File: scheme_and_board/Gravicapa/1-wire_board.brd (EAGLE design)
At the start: 33.3 x 12.1 mm, 10 parts, among them IC1 DS18B20

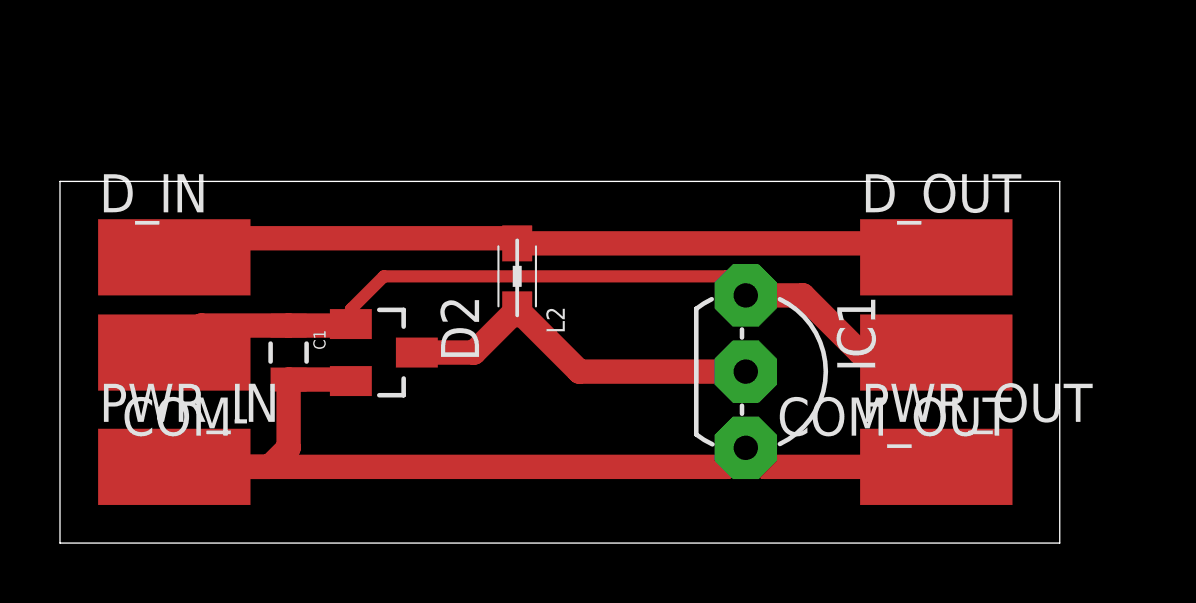
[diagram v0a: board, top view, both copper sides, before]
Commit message: �������� ����� ������������, ������� ��� ���������� � ������ ����������� ��� ������
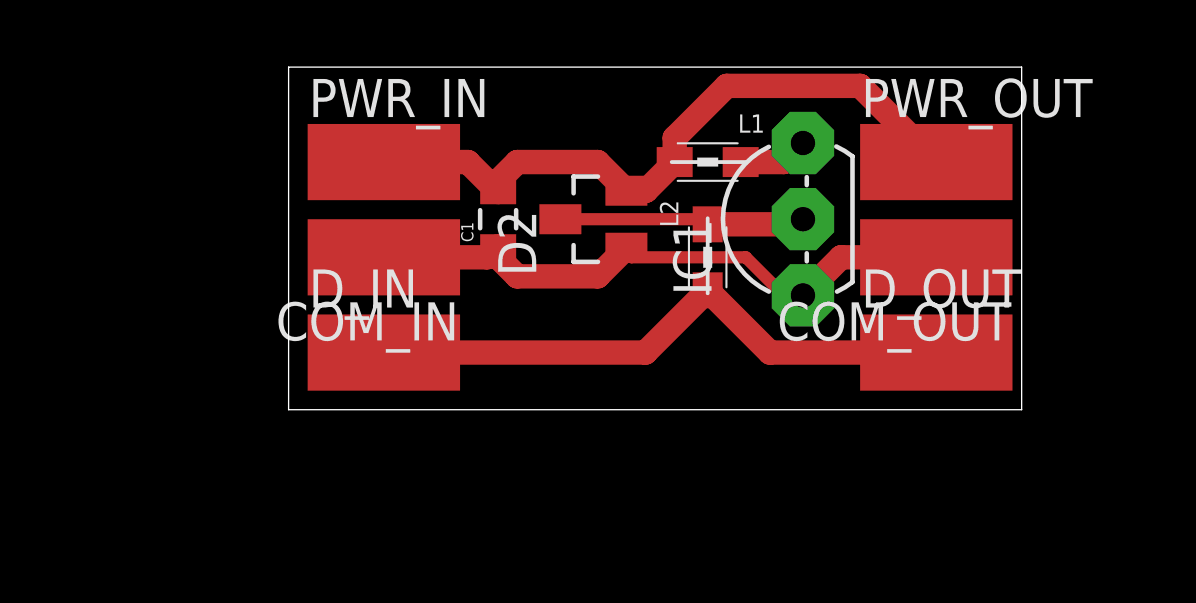
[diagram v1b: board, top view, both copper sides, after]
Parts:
- removed COM-: GND, wirepad:SMD2,54-5,08
- added COM_IN: GND, wirepad:SMD2,54-5,08
- added L1: BLM, wuerth-elektronik:0805
- moved PWR_IN 12.3 mm to (10.8, 12.7)
- moved PWR_OUT 10.2 mm to (29.2, 12.7)
- moved C1 8.28 mm to (14.6, 10.8), turned to 90 degrees
- moved D2 8.28 mm to (17.8, 10.8), turned to 90 degrees
- moved D_IN 7.67 mm to (10.8, 6.35)
- moved L2 6.38 mm to (21.6, 9.53), turned to 270 degrees
- moved IC1 5.43 mm to (24.8, 10.8), turned to 90 degrees
- moved COM_OUT 3.18 mm to (29.2, 9.53)
- moved D_OUT 3.18 mm to (29.2, 6.35)
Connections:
- new net N$4: C1.2, D2.2, L1.2, PWR_IN.1, PWR_OUT.1
- net N$3: now also COM_IN.1; no longer COM-.1
- net N$5: now also L1.1; no longer C1.2, D2.2, PWR_IN.1, PWR_OUT.1
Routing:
- net N$5: track 34.4 -> 2.34 mm
- net N$4: track 0.00 -> 22.8 mm
- net N$3: track 30.0 -> 21.1 mm
- net N$2: track 25.9 -> 20.1 mm
- net N$1: track 12.4 -> 8.23 mm
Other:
- board size 33.3 x 12.1 mm -> 24.4 x 11.4 mm
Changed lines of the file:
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@@
 <board>
 <plain>
-<wire x1="0" y1="0" x2="33.325" y2="0" width="0" layer="20"/>
-<wire x1="33.325" y1="0" x2="33.325" y2="12.055" width="0" layer="20"/>
-<wire x1="33.325" y1="12.055" x2="0" y2="12.055" width="0" layer="20"/>
-<wire x1="0" y1="12.055" x2="0" y2="0" width="0" layer="20"/>
+<wire x1="7.62" y1="4.445" x2="32.055" y2="4.445" width="0" layer="20"/>
+<wire x1="32.055" y1="4.445" x2="32.055" y2="15.865" width="0" layer="20"/>
+<wire x1="32.055" y1="15.865" x2="7.62" y2="15.865" width="0" layer="20"/>
+<wire x1="7.62" y1="15.865" x2="7.62" y2="4.445" width="0" layer="20"/>
 </plain>
 <attributes>
@@
 </autorouter>
 <elements>
-<element name="IC1" library="GravicapaLib" package="TO92-" value="DS18B20" x="22.86" y="5.715" rot="R270"/>
-<element name="L2" library="wuerth-elektronik" package="0805" value="BLM" x="15.24" y="8.89" rot="R90"/>
-<element name="D_IN" library="wirepad" package="SMD2,54-5,08" value="1-Wire" x="3.81" y="9.525" rot="R270"/>
-<element name="PWR_IN" library="wirepad" package="SMD2,54-5,08" value="VCC" x="3.81" y="2.54" rot="R270"/>
-<element name="COM-" library="wirepad" package="SMD2,54-5,08" value="GND" x="3.81" y="6.35" rot="R90"/>
-<element name="PWR_OUT" library="wirepad" package="SMD2,54-5,08" value="VCC" x="29.21" y="2.54" rot="R270"/>
-<element name="D_OUT" library="wirepad" package="SMD2,54-5,08" value="1-Wire" x="29.21" y="9.525" rot="R270"/>
-<element name="COM_OUT" library="wirepad" package="SMD2,54-5,08" value="GND" x="29.21" y="6.35" rot="R90"/>
-<element name="D2" library="GravicapaLib" package="SOT23" value="BAV199" x="10.795" y="6.35" rot="R270"/>
-<element name="C1" library="GravicapaLib" package="0805" value="0.1uF" x="7.62" y="6.35" rot="R270"/>
+<element name="IC1" library="GravicapaLib" package="TO92-" value="DS18B20" x="24.765" y="10.795" rot="R90"/>
+<element name="L2" library="wuerth-elektronik" package="0805" value="BLM" x="21.59" y="9.525" rot="R270"/>
+<element name="D_IN" library="wirepad" package="SMD2,54-5,08" value="1-Wire" x="10.795" y="6.35" rot="R270"/>
+<element name="PWR_IN" library="wirepad" package="SMD2,54-5,08" value="VCC" x="10.795" y="12.7" rot="R270"/>
+<element name="COM_IN" library="wirepad" package="SMD2,54-5,08" value="GND" x="10.795" y="9.525" rot="R90"/>
+<element name="PWR_OUT" library="wirepad" package="SMD2,54-5,08" value="VCC" x="29.21" y="12.7" rot="R270"/>
+<element name="D_OUT" library="wirepad" package="SMD2,54-5,08" value="1-Wire" x="29.21" y="6.35" rot="R270"/>
+<element name="COM_OUT" library="wirepad" package="SMD2,54-5,08" value="GND" x="29.21" y="9.525" rot="R90"/>
+<element name="D2" library="GravicapaLib" package="SOT23" value="BAV199" x="17.78" y="10.795" rot="R90"/>
+<element name="C1" library="GravicapaLib" package="0805" value="0.1uF" x="14.605" y="10.795" rot="R90"/>
+<element name="L1" library="wuerth-elektronik" package="0805" value="BLM" x="21.59" y="12.7" rot="R180"/>
 </elements>
 <signals>
@@
 <contactref element="IC1" pad="2"/>
 <contactref element="D2" pad="3"/>
-<wire x1="22.86" y1="5.715" x2="17.315" y2="5.715" width="0.8128" layer="1"/>
-<wire x1="17.315" y1="5.715" x2="15.24" y2="7.79" width="0.8128" layer="1"/>
-<wire x1="11.895" y1="6.35" x2="13.8" y2="6.35" width="0.8128" layer="1"/>
-<wire x1="13.8" y1="6.35" x2="15.24" y2="7.79" width="0.8128" layer="1"/>
+<wire x1="16.68" y1="10.795" x2="21.42" y2="10.795" width="0.4064" layer="1"/>
+<wire x1="21.42" y1="10.795" x2="21.59" y2="10.625" width="0.4064" layer="1"/>
+<wire x1="21.59" y1="10.625" x2="24.595" y2="10.625" width="0.8128" layer="1"/>
+<wire x1="24.595" y1="10.625" x2="24.765" y2="10.795" width="0.4064" layer="1"/>
 </signal>
 <signal name="N$5">
-<contactref element="PWR_OUT" pad="1"/>
 <contactref element="IC1" pad="3"/>
-<wire x1="22.86" y1="3.175" x2="23.495" y2="2.54" width="0.8128" layer="1"/>
-<wire x1="23.495" y1="2.54" x2="29.21" y2="2.54" width="0.8128" layer="1"/>
-<contactref element="PWR_IN" pad="1"/>
-<contactref element="D2" pad="2"/>
-<contactref element="C1" pad="2"/>
-<wire x1="7.62" y1="5.45" x2="9.645" y2="5.45" width="0.8128" layer="1"/>
-<wire x1="9.645" y1="5.45" x2="9.695" y2="5.4" width="0.8128" layer="1"/>
-<wire x1="3.81" y1="2.54" x2="22.225" y2="2.54" width="0.8128" layer="1"/>
-<wire x1="22.225" y1="2.54" x2="22.86" y2="3.175" width="0.8128" layer="1"/>
-<wire x1="3.81" y1="2.54" x2="6.985" y2="2.54" width="0.8128" layer="1"/>
-<wire x1="6.985" y1="2.54" x2="7.62" y2="3.175" width="0.8128" layer="1"/>
-<wire x1="7.62" y1="3.175" x2="7.62" y2="5.45" width="0.8128" layer="1"/>
+<contactref element="L1" pad="1"/>
+<wire x1="22.69" y1="12.7" x2="24.13" y2="12.7" width="0.8128" layer="1"/>
+<wire x1="24.13" y1="12.7" x2="24.765" y2="13.335" width="0.8128" layer="1"/>
 </signal>
 <signal name="N$3">
-<contactref element="COM-" pad="1"/>
+<contactref element="COM_IN" pad="1"/>
 <contactref element="IC1" pad="1"/>
 <contactref element="COM_OUT" pad="1"/>
 <contactref element="D2" pad="1"/>
 <contactref element="C1" pad="1"/>
-<wire x1="5.08" y1="6.35" x2="5.715" y2="6.985" width="1.016" layer="1"/>
-<wire x1="29.21" y1="6.35" x2="26.67" y2="6.35" width="0.8128" layer="1"/>
-<wire x1="26.67" y1="6.35" x2="24.765" y2="8.255" width="0.8128" layer="1"/>
-<wire x1="24.765" y1="8.255" x2="22.86" y2="8.255" width="0.8128" layer="1"/>
-<wire x1="3.81" y1="6.35" x2="5.08" y2="6.35" width="0.8128" layer="1"/>
-<wire x1="7.62" y1="7.25" x2="4.71" y2="7.25" width="0.8128" layer="1"/>
-<wire x1="4.71" y1="7.25" x2="3.81" y2="6.35" width="0.8128" layer="1"/>
-<wire x1="7.62" y1="7.25" x2="9.645" y2="7.25" width="0.8128" layer="1"/>
-<wire x1="9.645" y1="7.25" x2="9.695" y2="7.3" width="0.8128" layer="1"/>
-<wire x1="9.695" y1="7.3" x2="9.695" y2="7.79" width="0.4064" layer="1"/>
-<wire x1="9.695" y1="7.79" x2="10.795" y2="8.89" width="0.4064" layer="1"/>
-<wire x1="10.795" y1="8.89" x2="22.225" y2="8.89" width="0.4064" layer="1"/>
-<wire x1="22.225" y1="8.89" x2="22.86" y2="8.255" width="0.4064" layer="1"/>
+<wire x1="10.795" y1="9.525" x2="14.235" y2="9.525" width="0.8128" layer="1"/>
+<wire x1="14.235" y1="9.525" x2="14.605" y2="9.895" width="0.8128" layer="1"/>
+<wire x1="14.605" y1="9.895" x2="14.605" y2="9.525" width="0.4064" layer="1"/>
+<wire x1="14.605" y1="9.525" x2="15.24" y2="8.89" width="0.8128" layer="1"/>
+<wire x1="15.24" y1="8.89" x2="17.925" y2="8.89" width="0.8128" layer="1"/>
+<wire x1="17.925" y1="8.89" x2="18.88" y2="9.845" width="0.8128" layer="1"/>
+<wire x1="24.765" y1="8.255" x2="26.035" y2="9.525" width="0.8128" layer="1"/>
+<wire x1="26.035" y1="9.525" x2="29.21" y2="9.525" width="0.8128" layer="1"/>
+<wire x1="24.765" y1="8.255" x2="24.13" y2="8.255" width="0.4064" layer="1"/>
+<wire x1="24.13" y1="8.255" x2="22.86" y2="9.525" width="0.4064" layer="1"/>
+<wire x1="22.86" y1="9.525" x2="19.05" y2="9.525" width="0.4064" layer="1"/>
+<wire x1="19.05" y1="9.525" x2="18.73" y2="9.845" width="0.4064" layer="1"/>
+<wire x1="18.73" y1="9.845" x2="18.88" y2="9.845" width="0.4064" layer="1"/>
 </signal>
 <signal name="N$2">
@@
 <contactref element="L2" pad="2"/>
 <contactref element="D_OUT" pad="1"/>
-<wire x1="3.81" y1="9.525" x2="5.08" y2="9.525" width="0.8128" layer="1"/>
-<wire x1="5.08" y1="9.525" x2="5.715" y2="10.16" width="0.8128" layer="1"/>
-<wire x1="5.715" y1="10.16" x2="15.07" y2="10.16" width="0.8128" layer="1"/>
-<wire x1="15.07" y1="10.16" x2="15.24" y2="9.99" width="0.8128" layer="1"/>
-<wire x1="15.24" y1="9.99" x2="28.745" y2="9.99" width="0.8128" layer="1"/>
-<wire x1="28.745" y1="9.99" x2="29.21" y2="9.525" width="0.8128" layer="1"/>
+<wire x1="10.795" y1="6.35" x2="19.515" y2="6.35" width="0.8128" layer="1"/>
+<wire x1="19.515" y1="6.35" x2="21.59" y2="8.425" width="0.8128" layer="1"/>
+<wire x1="21.59" y1="8.425" x2="23.665" y2="6.35" width="0.8128" layer="1"/>
+<wire x1="23.665" y1="6.35" x2="29.21" y2="6.35" width="0.8128" layer="1"/>
+</signal>
+<signal name="N$4">
+<contactref element="PWR_IN" pad="1"/>
+<contactref element="D2" pad="2"/>
+<contactref element="C1" pad="2"/>
+<contactref element="L1" pad="2"/>
+<wire x1="10.795" y1="12.7" x2="13.6" y2="12.7" width="0.8128" layer="1"/>
+<wire x1="13.6" y1="12.7" x2="14.605" y2="11.695" width="0.8128" layer="1"/>
+<wire x1="14.605" y1="11.695" x2="14.605" y2="12.065" width="0.4064" layer="1"/>
+<wire x1="14.605" y1="12.065" x2="15.24" y2="12.7" width="0.8128" layer="1"/>
+<wire x1="15.24" y1="12.7" x2="17.925" y2="12.7" width="0.8128" layer="1"/>
+<wire x1="17.925" y1="12.7" x2="18.88" y2="11.745" width="0.8128" layer="1"/>
+<wire x1="18.88" y1="11.745" x2="19.535" y2="11.745" width="0.8128" layer="1"/>
+<wire x1="19.535" y1="11.745" x2="20.49" y2="12.7" width="0.8128" layer="1"/>
+<contactref element="PWR_OUT" pad="1"/>
+<wire x1="29.21" y1="12.7" x2="26.67" y2="15.24" width="0.8128" layer="1"/>
+<wire x1="26.67" y1="15.24" x2="22.225" y2="15.24" width="0.8128" layer="1"/>
+<wire x1="22.225" y1="15.24" x2="20.49" y2="13.505" width="0.8128" layer="1"/>
+<wire x1="20.49" y1="13.505" x2="20.49" y2="12.7" width="0.8128" layer="1"/>
 </signal>
 </signals>
